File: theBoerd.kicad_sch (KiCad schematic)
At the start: 170 parts, among them J2 USB_C_Receptacle, U1 Elite-C

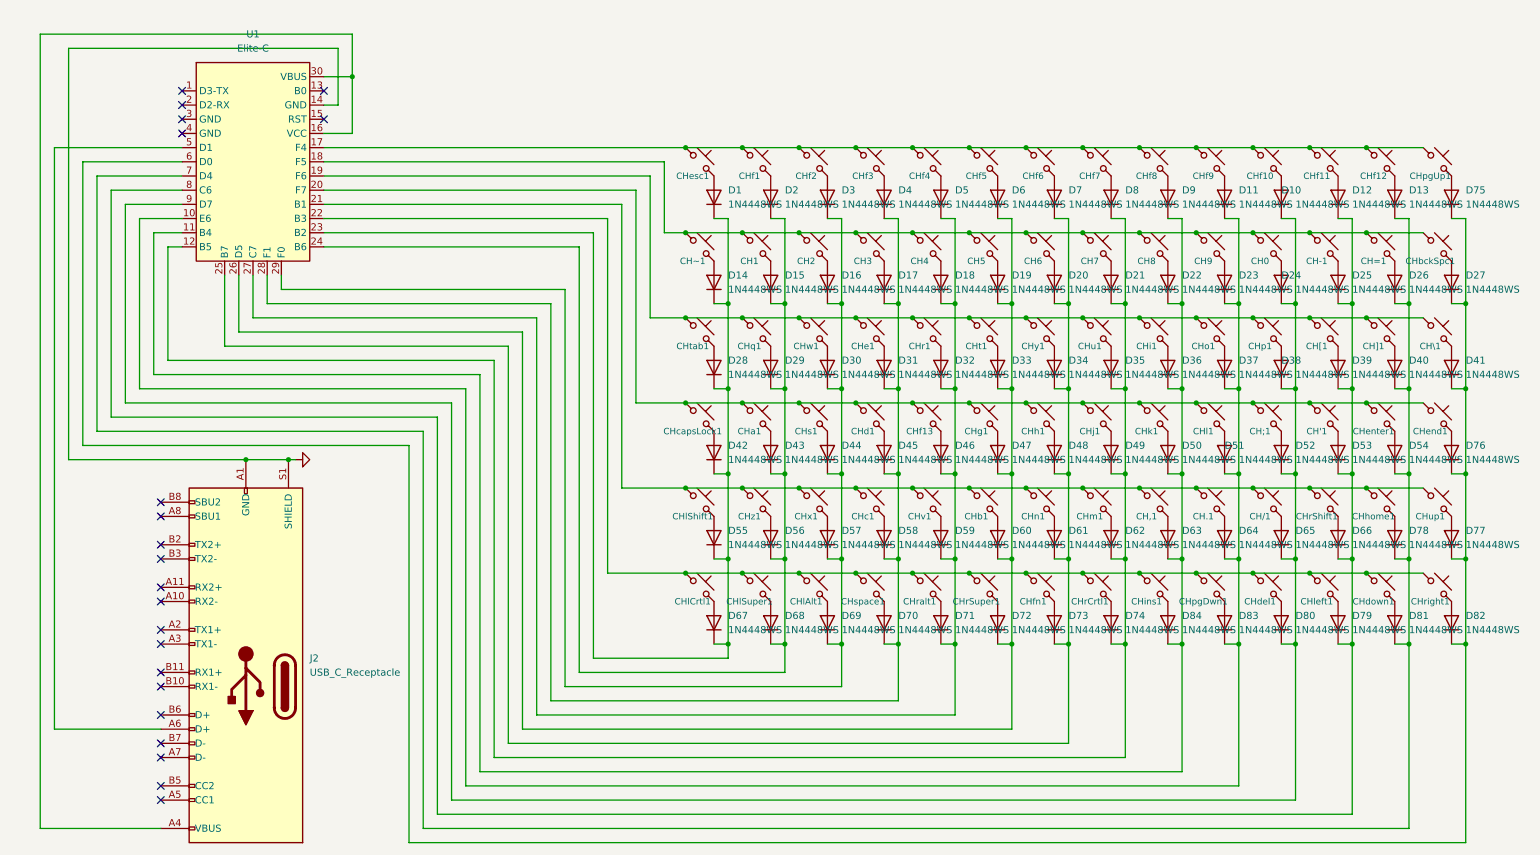
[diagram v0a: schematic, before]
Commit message: Project Restart
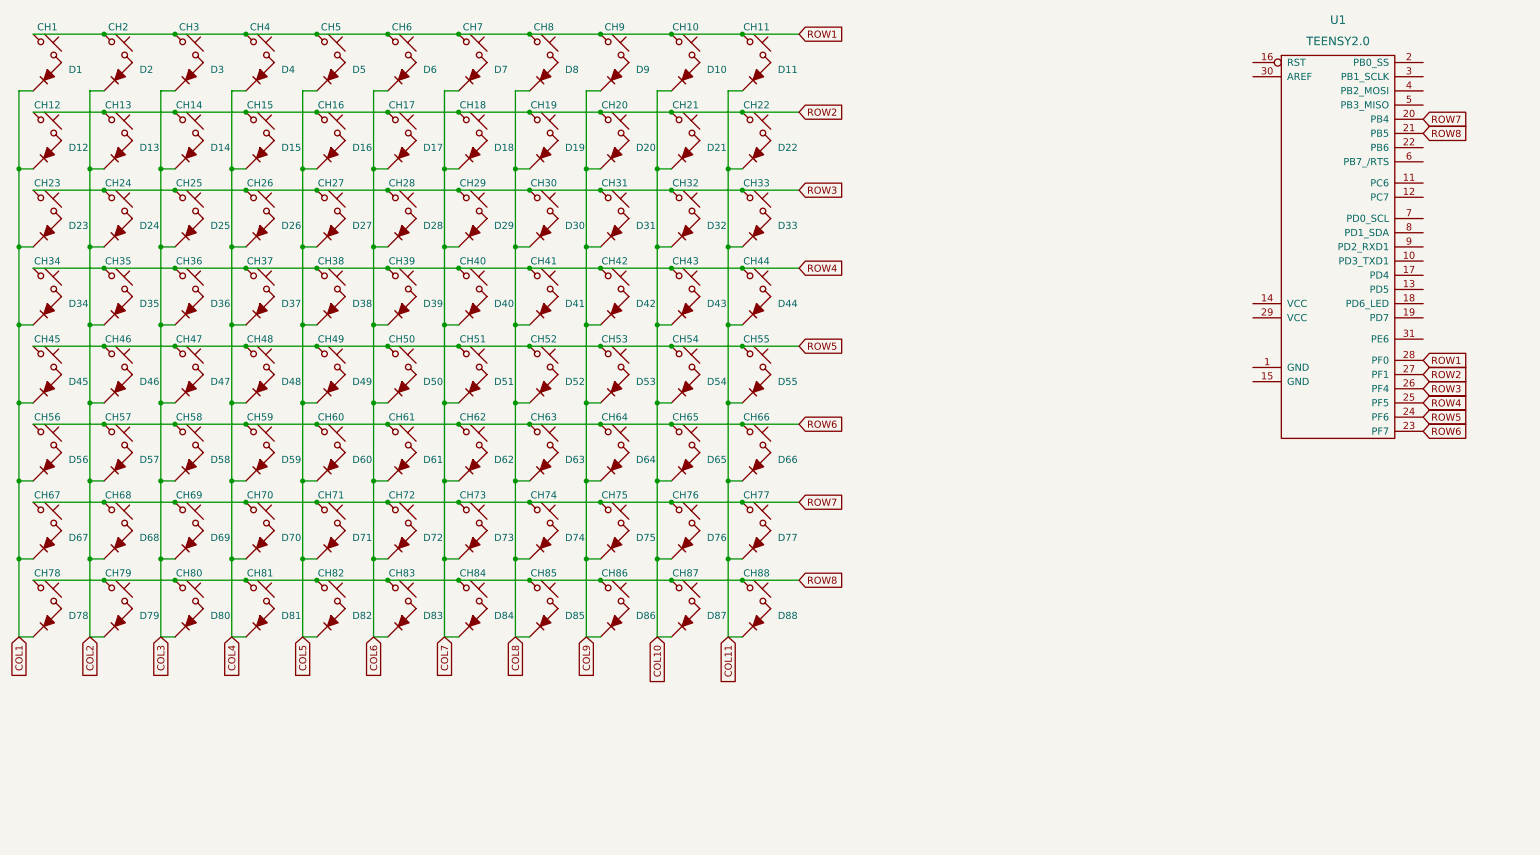
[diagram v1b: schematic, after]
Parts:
- removed CH'1, CH,1, CH-1, CH.1, CH/1, CH0, CH;1, CH=1, CH[1, CH\1, CH]1, CHa1, CHb1, CHbckSpc1, CHc1, CHcapsLock1, CHd1, CHdel1, CHdown1, CHe1, CHend1, CHenter1, CHesc1, CHf1, CHf10, CHf11, CHf12, CHf13, CHf2, CHf3, CHf4, CHf5, CHf6, CHf7, CHf8, CHf9, CHfn1, CHg1, CHh1, CHhome1, CHi1, CHins1, CHj1, CHk1, CHl1, CHlAlt1, CHlCrtl1, CHlShift1, CHlSuper1, CHleft1, CHm1, CHn1, CHo1, CHp1, CHpgDwn1, CHpgUp1, CHq1, CHr1, CHrCrtl1, CHrShift1, CHrSuper1, CHralt1, CHright1, CHs1, CHspace1, CHt1, CHtab1, CHu1, CHup1, CHv1, CHw1, CHx1, CHy1, CHz1, CH~1: ~, Gateron_KS33_Hotswap:Gateron-KS33-Hotswap-1U, symbol marbastlib-gateron_lp:KS33_SW_HS_KS-2P02B01-02
- removed D1, D10, D11, D12, D13, D14, D15, D16, D17, D18, D19, D2, D20, D21, D22, D23, D24, D25, D26, D27, D28, D29, D3, D30, D31, D32, D33, D34, D35, D36, D37, D38, D39, D4, D40, D41, D42, D43, D44, D45, D46, D47, D48, D49, D5, D50, D51, D52, D53, D54, D55, D56, D57, D58, D59, D6, D60, D61, D62, D63, D64, D65, D66, D67, D68, D69, D7, D70, D71, D72, D73, D74, D75, D76, D77, D78, D79, D8, D80, D81, D82, D83, D84, D9: 1N4448WS, Diode_SMD:D_SOD-323, symbol Diode:1N4448WS
- removed J2: USB_C_Receptacle, Connector_USB:USB_C_Receptacle_HRO_TYPE-C-31-M-12, symbol Connector:USB_C_Receptacle
- removed U1: Elite-C, TerminalBlock_Dinkle:TerminalBlock_Dinkle_DT-55-B01X-30_P10.00mm, symbol marbastlib-promicroish:Elite-C
- added CH10, CH11, CH12, CH13, CH14, CH15, CH16, CH17, CH18, CH19, CH20, CH21, CH22, CH23, CH24, CH25, CH26, CH27, CH28, CH29, CH30, CH31, CH32, CH33, CH34, CH35, CH36, CH37, CH38, CH39, CH40, CH41, CH42, CH43, CH44, CH45, CH46, CH47, CH48, CH49, CH50, CH51, CH52, CH53, CH54, CH55, CH56, CH57, CH58, CH59, CH60, CH61, CH62, CH63, CH64, CH65, CH66, CH67, CH68, CH69, CH70, CH71, CH72, CH73, CH74, CH75, CH76, CH77, CH78, CH79, CH80, CH81, CH82, CH83, CH84, CH85, CH86, CH87, CH88: KS33_SW_HS, PCM_marbastlib-gateron_lp:SW_KS33_HS_KS-2P02B01-02_HS_1u, symbol marbastlib-gateron_lp:KS33_SW_HS_KS-2P02B01-02
- added D1, D10, D11, D12, D13, D14, D15, D16, D17, D18, D19, D2, D20, D21, D22, D23, D24, D25, D26, D27, D28, D29, D3, D30, D31, D32, D33, D34, D35, D36, D37, D38, D39, D4, D40, D41, D42, D43, D44, D45, D46, D47, D48, D49, D5, D50, D51, D52, D53, D54, D55, D56, D57, D58, D59, D6, D60, D61, D62, D63, D64, D65, D66, D67, D68, D69, D7, D70, D71, D72, D73, D74, D75, D76, D77, D78, D79, D8, D80, D81, D82, D83, D84, D85, D86, D87, D88, D9: D_45deg_Filled, symbol Device:D_45deg_Filled
- added U1: TEENSY2.0, symbol component:TEENSY2.0
- CH1, CH2, CH3, CH4, CH5, CH6, CH7, CH8, CH9: value ~ -> KS33_SW_HS; footprint Gateron_KS33_Hotswap:Gateron-KS33-Hotswap-1U -> PCM_marbastlib-gateron_lp:SW_KS33_HS_KS-2P02B01-02_HS_1u
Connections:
- net at CH3.2: now also D3.2 (A)
- net ROW1: now reaches CH1.1, CH2.1, CH3.1, CH4.1, CH5.1, CH6.1, CH7.1, CH8.1, CH9.1
- net ROW1: now also CH10.1, CH11.1, U1.28 (PF0)
- net at CH4.2: now also D4.2 (A)
- net at CH7.2: now also D7.2 (A)
- net at CH5.2: now also D5.2 (A)
- net at CH9.2: now also D9.2 (A)
- net at CH8.2: now also D8.2 (A)
- net at CH2.2: now also D2.2 (A)
- net at CH6.2: now also D6.2 (A)
- net at CH1.2: now also D1.2 (A)
- new net: CH48.2, D48.2 (A)
- new net: CH45.2, D45.2 (A)
- new net: CH20.2, D20.2 (A)
- new net: CH64.2, D64.2 (A)
- new net: CH31.2, D31.2 (A)
- new net: CH16.2, D16.2 (A)
- new net: CH57.2, D57.2 (A)
- new net: CH86.2, D86.2 (A)
- new net: CH18.2, D18.2 (A)
- new net: CH22.2, D22.2 (A)
- new net: CH75.2, D75.2 (A)
- new net: CH88.2, D88.2 (A)
- new net: CH71.2, D71.2 (A)
- new net: CH51.2, D51.2 (A)
- new net: CH83.2, D83.2 (A)
- new net: CH76.2, D76.2 (A)
- new net: CH21.2, D21.2 (A)
- new net: CH66.2, D66.2 (A)
- new net: CH24.2, D24.2 (A)
- new net: CH27.2, D27.2 (A)
- new net: CH10.2, D10.2 (A)
- new net: CH77.2, D77.2 (A)
- new net: CH80.2, D80.2 (A)
- new net: CH67.2, D67.2 (A)
- new net: CH84.2, D84.2 (A)
- new net: CH38.2, D38.2 (A)
- new net: CH63.2, D63.2 (A)
- new net: CH34.2, D34.2 (A)
- new net: CH60.2, D60.2 (A)
- new net: CH78.2, D78.2 (A)
- new net: CH52.2, D52.2 (A)
- new net: CH72.2, D72.2 (A)
- new net: CH50.2, D50.2 (A)
- new net: CH29.2, D29.2 (A)
- new net: CH40.2, D40.2 (A)
- new net: CH47.2, D47.2 (A)
- new net: CH43.2, D43.2 (A)
- new net: CH39.2, D39.2 (A)
- new net: CH36.2, D36.2 (A)
- new net: CH23.2, D23.2 (A)
- new net: CH44.2, D44.2 (A)
- new net: CH26.2, D26.2 (A)
- new net: CH70.2, D70.2 (A)
- new net: CH37.2, D37.2 (A)
- new net: CH49.2, D49.2 (A)
- new net: CH15.2, D15.2 (A)
- new net: CH81.2, D81.2 (A)
- new net: CH61.2, D61.2 (A)
- new net: CH58.2, D58.2 (A)
- new net: CH11.2, D11.2 (A)
- new net: CH25.2, D25.2 (A)
- new net: CH56.2, D56.2 (A)
- new net: CH65.2, D65.2 (A)
- new net: CH62.2, D62.2 (A)
- new net: CH17.2, D17.2 (A)
- new net: CH55.2, D55.2 (A)
- new net: CH33.2, D33.2 (A)
- new net: CH46.2, D46.2 (A)
- new net: CH73.2, D73.2 (A)
- new net: CH82.2, D82.2 (A)
- new net: CH42.2, D42.2 (A)
- new net: CH74.2, D74.2 (A)
- new net: CH35.2, D35.2 (A)
- new net: CH30.2, D30.2 (A)
- new net: CH19.2, D19.2 (A)
- new net: CH32.2, D32.2 (A)
- new net: CH68.2, D68.2 (A)
- new net: CH87.2, D87.2 (A)
- new net: CH54.2, D54.2 (A)
- new net: CH13.2, D13.2 (A)
- new net: CH69.2, D69.2 (A)
- new net: CH85.2, D85.2 (A)
- new net: CH79.2, D79.2 (A)
- new net: CH53.2, D53.2 (A)
- new net: CH12.2, D12.2 (A)
- new net: CH28.2, D28.2 (A)
- new net: CH59.2, D59.2 (A)
- new net: CH14.2, D14.2 (A)
- new net: CH41.2, D41.2 (A)
- new net COL1: D1.1 (K), D12.1 (K), D23.1 (K), D34.1 (K), D45.1 (K), D56.1 (K), D67.1 (K), D78.1 (K)
- new net COL10: D10.1 (K), D21.1 (K), D32.1 (K), D43.1 (K), D54.1 (K), D65.1 (K), D76.1 (K), D87.1 (K)
- new net COL11: D11.1 (K), D22.1 (K), D33.1 (K), D44.1 (K), D55.1 (K), D66.1 (K), D77.1 (K), D88.1 (K)
- new net COL2: D13.1 (K), D2.1 (K), D24.1 (K), D35.1 (K), D46.1 (K), D57.1 (K), D68.1 (K), D79.1 (K)
- new net COL3: D14.1 (K), D25.1 (K), D3.1 (K), D36.1 (K), D47.1 (K), D58.1 (K), D69.1 (K), D80.1 (K)
- new net COL4: D15.1 (K), D26.1 (K), D37.1 (K), D4.1 (K), D48.1 (K), D59.1 (K), D70.1 (K), D81.1 (K)
- new net COL5: D16.1 (K), D27.1 (K), D38.1 (K), D49.1 (K), D5.1 (K), D60.1 (K), D71.1 (K), D82.1 (K)
- new net COL6: D17.1 (K), D28.1 (K), D39.1 (K), D50.1 (K), D6.1 (K), D61.1 (K), D72.1 (K), D83.1 (K)
- new net COL7: D18.1 (K), D29.1 (K), D40.1 (K), D51.1 (K), D62.1 (K), D7.1 (K), D73.1 (K), D84.1 (K)
- new net COL8: D19.1 (K), D30.1 (K), D41.1 (K), D52.1 (K), D63.1 (K), D74.1 (K), D8.1 (K), D85.1 (K)
- new net COL9: D20.1 (K), D31.1 (K), D42.1 (K), D53.1 (K), D64.1 (K), D75.1 (K), D86.1 (K), D9.1 (K)
- new net ROW2: CH12.1, CH13.1, CH14.1, CH15.1, CH16.1, CH17.1, CH18.1, CH19.1, CH20.1, CH21.1, CH22.1, U1.27 (PF1)
- new net ROW3: CH23.1, CH24.1, CH25.1, CH26.1, CH27.1, CH28.1, CH29.1, CH30.1, CH31.1, CH32.1, CH33.1, U1.26 (PF4)
- new net ROW4: CH34.1, CH35.1, CH36.1, CH37.1, CH38.1, CH39.1, CH40.1, CH41.1, CH42.1, CH43.1, CH44.1, U1.25 (PF5)
- new net ROW5: CH45.1, CH46.1, CH47.1, CH48.1, CH49.1, CH50.1, CH51.1, CH52.1, CH53.1, CH54.1, CH55.1, U1.24 (PF6)
- new net ROW6: CH56.1, CH57.1, CH58.1, CH59.1, CH60.1, CH61.1, CH62.1, CH63.1, CH64.1, CH65.1, CH66.1, U1.23 (PF7)
- new net ROW7: CH67.1, CH68.1, CH69.1, CH70.1, CH71.1, CH72.1, CH73.1, CH74.1, CH75.1, CH76.1, CH77.1, U1.20 (PB4)
- new net ROW8: CH78.1, CH79.1, CH80.1, CH81.1, CH82.1, CH83.1, CH84.1, CH85.1, CH86.1, CH87.1, CH88.1, U1.21 (PB5)
- no-connect marks 21 -> 0
